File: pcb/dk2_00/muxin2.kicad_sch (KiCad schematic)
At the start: 7 parts, among them J12 AudioJack2_SwitchT, U15 MCP6002-xSN, U6 74HC4051

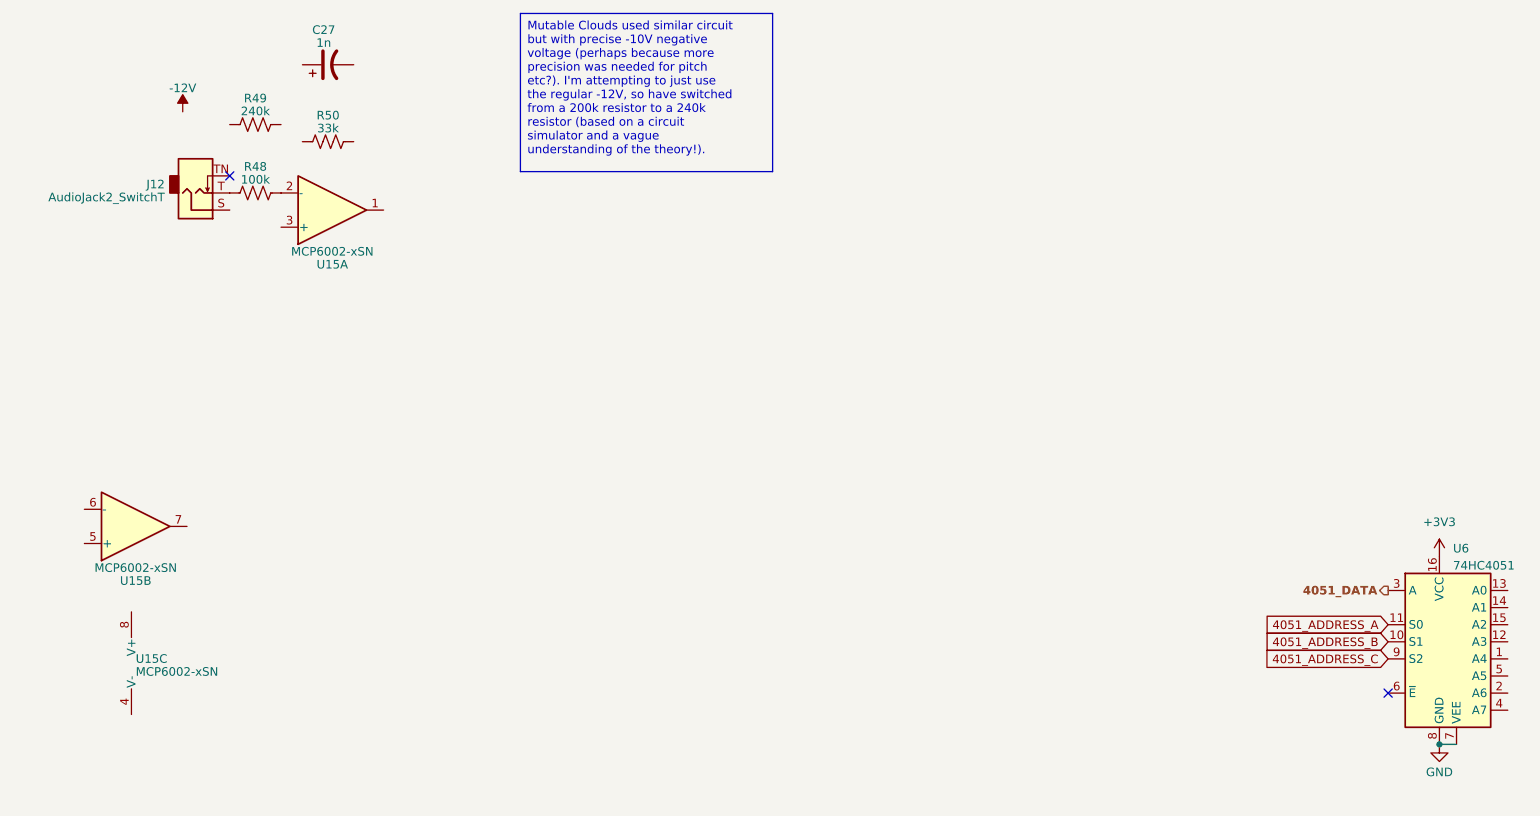
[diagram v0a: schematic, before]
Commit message: tidying up, getting close!
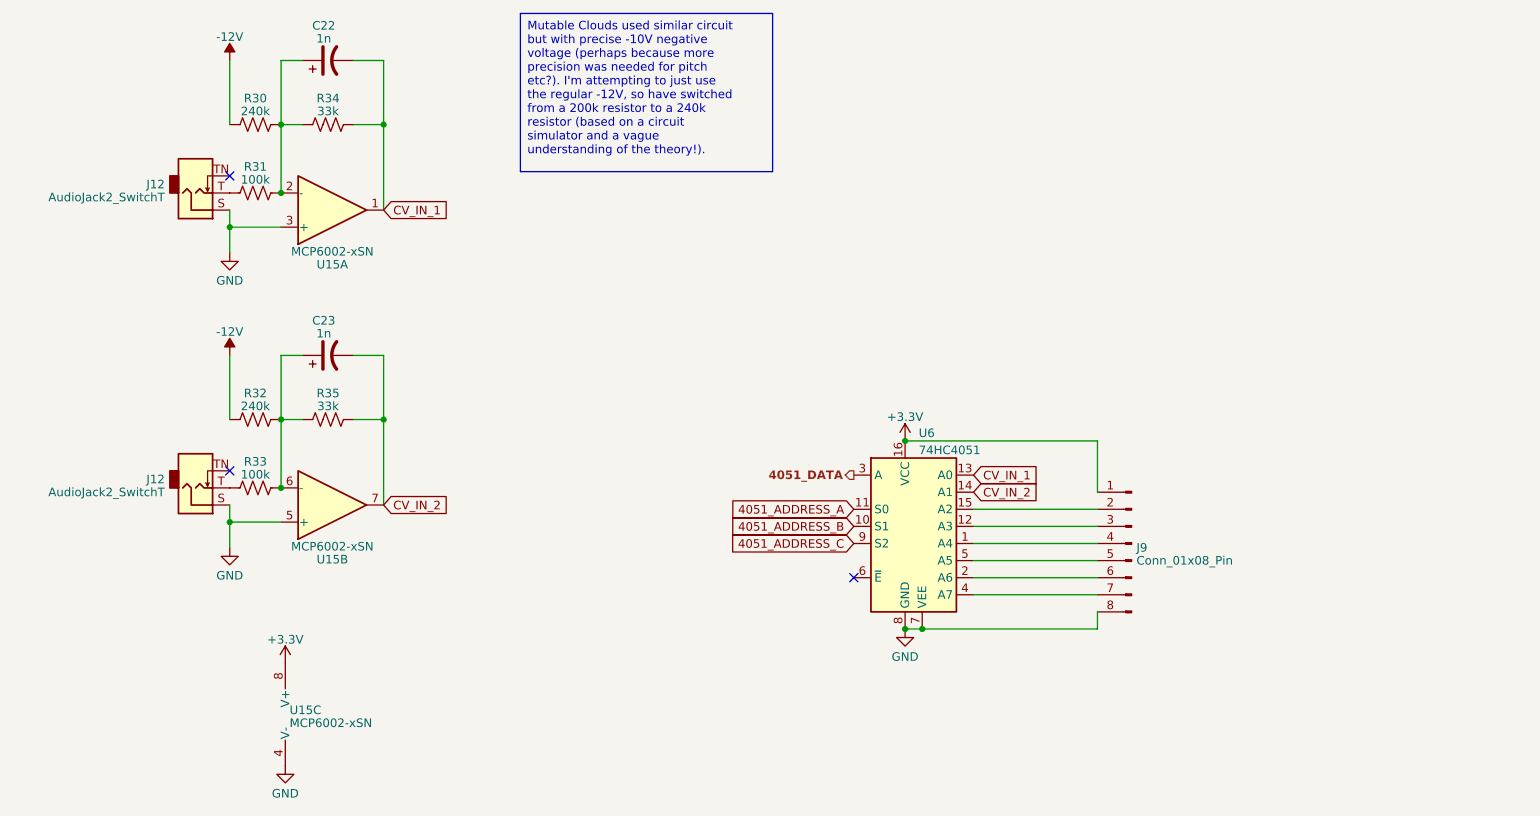
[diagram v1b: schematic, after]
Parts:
- added C23: 1n, symbol Device:C_Polarized_US
- added J12: AudioJack2_SwitchT, AudioJacks:Jack_3.5mm_QingPu_WQP-PJ398SM_Vertical, symbol Connector_Audio:AudioJack2_SwitchT
- added J9: Conn_01x08_Pin, symbol Connector:Conn_01x08_Pin
- added R32: 240k, symbol Device:R_US
- added R33: 100k, symbol Device:R_US
- added R35: 33k, symbol Device:R_US
- renumbered C27 to C22, R49 to R30, R48 to R31, R50 to R34
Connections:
- net +3V3 is gone; now on net +3.3V: U6.16 (VCC)
- net -12V: now also R30.1, R32.1
- net GND: now also J12.S, U15.3 (+), U15.4 (V-), U15.5 (+), J12.S, J9.8 (Pin_8)
- net at C22.1: now also R30.2, R31.2, R34.1, U15.2 (-)
- net CV_IN_1: now reaches C22.2
- net CV_IN_1: now also R34.2, U15.1, U6.13 (A0)
- net at U15.6 (-): now also C23.1, R32.2, R33.2, R35.1
- net CV_IN_2: now reaches U15.7
- net CV_IN_2: now also U6.14 (A1), C23.2, R35.2
- net +3.3V: now reaches U15.8 (V+)
- net +3.3V: now also J9.1 (Pin_1)
- net at U6.1 (A4): now also J9.4 (Pin_4)
- net at U6.12 (A3): now also J9.3 (Pin_3)
- net at U6.15 (A2): now also J9.2 (Pin_2)
- net at U6.2 (A6): now also J9.6 (Pin_6)
- net at U6.4 (A7): now also J9.7 (Pin_7)
- net at U6.5 (A5): now also J9.5 (Pin_5)
- new net: J12.T, R33.1
- no-connect marks 2 -> 3
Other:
- moved on the sheet: C22, R34, U15B, U15C
